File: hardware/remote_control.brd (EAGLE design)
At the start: 19.5 x 100 mm, 52 parts, among them IC1 MCP4726, IC3 REG1117, IC4 TL072D, IC5 LM4041A12DBZ

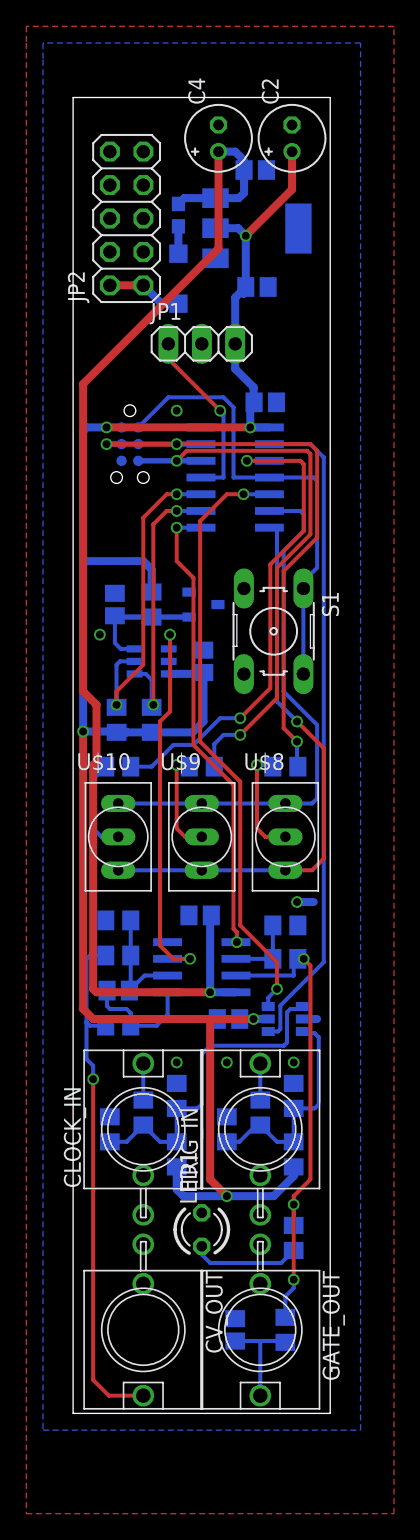
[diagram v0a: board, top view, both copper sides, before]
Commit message: rfsw
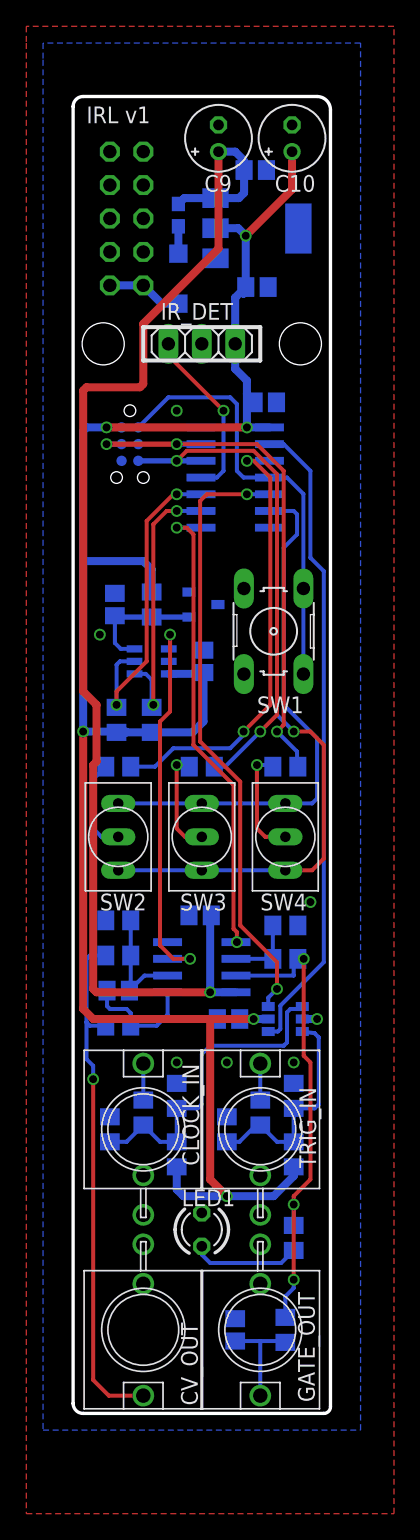
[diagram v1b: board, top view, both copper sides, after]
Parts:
- removed C11, C12: (no value), resistor:C0805
- removed D9: TS4148, jason_eagle6:D0805
- added C3: (no value), resistor:C0805
- added D2: TS4148, jason_eagle6:D0805
- added R3: (no value), rcl:R0805
- C10, C9: device resistor:C0805 -> resistor:E2-5
- C2, C4: device resistor:E2-5 -> resistor:C0805
- IC1: value MCP4726 -> REG1117; device jasons_stuff:SOT23-6 -> burr-brown:SOT223
- IC3: value REG1117 -> LM4041A12DBZ; device burr-brown:SOT223 -> texas:DBZ_R-PDSO-G3
- IC4: value TL072D -> MCP4726; device linear:SO08 -> jasons_stuff:SOT23-6
- IC5: value LM4041A12DBZ -> TL072D; device texas:DBZ_R-PDSO-G3 -> linear:SO08
- R1: value (none) -> 3k
- R14: value 3k -> (none)
- R8: device rcl:R0805 -> resistor:C0805
- moved C10 90.7 mm to (20.2, 96.9), flipped to the top, turned to 90 degrees
- moved C8 70.5 mm to (15.9, 6.35), turned to 270 degrees
- moved C1 64.5 mm to (17.4, 94.5), turned to 0 degrees
- moved R1 49.3 mm to (9.53, 61.5), turned to 90 degrees
- moved R14 49.3 mm to (20.3, 13.3), turned to 270 degrees
- moved R15 48.1 mm to (19.7, 6.35), turned to 90 degrees
- moved C6 47.9 mm to (13.2, 37.8)
- moved C5 37.5 mm to (13.5, 57.1), turned to 90 degrees
- moved C4 36.3 mm to (6.73, 61.5), flipped to the bottom, turned to 270 degrees
- moved C9 36.3 mm to (14.6, 96.9), flipped to the top, turned to 90 degrees
- moved IC1 33.9 mm to (17.5, 90.0), turned to 90 degrees
- moved D4 32.3 mm to (6.99, 49.1), turned to 180 degrees
- moved D7 30.6 mm to (11.4, 19.7), turned to 270 degrees
- moved IC3 28.9 mm to (13.5, 61.5)
- moved R8 28.7 mm to (6.99, 32.1), turned to 0 degrees
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- renumbered FB1 to L1, JP1 to IR_DET, R16 to R2, S1 to SW1, U$1 to IC2, U$10 to SW2, U$6 to IC6, U$8 to SW4, U$9 to SW3
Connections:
- net +12V: now also C1.2, C6.1, C9.+, IC1.3, IC5.8; no longer C12.1, C4.+, C5.2, IC3.3, IC4.8
- net CV_OUT: now also IC4.1, IC5.3; no longer IC1.1, IC4.3
- net GATE_OUT: now also IC5.5; no longer IC4.5
- net GND: now also C10.-, C2.1, C3.1, C4.1, C5.2, C6.2, C7.1, C9.-, D6.A, D8.A, IC1.1, IC3.2, IC4.2, IC5.4, R10.2, R12.2, R4.2, R6.2; no longer C10.1, C12.2, C2.-, C4.-, C5.1, C6.1, C7.2, C9.1, D3.A, D5.A, IC1.2, IC3.1, IC4.4, IC5.2, R13.2, R5.2, R7.2, R9.2
- net N$10: now also R11.1; no longer R4.1
- net N$11: now also D2.A; no longer D7.A
- net N$13: now also IC5.7, R14.1, R15.2, R5.1; no longer IC4.7, R1.1, R10.1, R8.2
- net N$14: now also D7.A, D8.K, R12.1, R13.2; no longer D5.K, D6.A, R6.2, R7.1
- net N$15: now also D3.A; no longer D8.A
- net N$16: now also C8.2, R15.1; no longer C10.2, R8.1
- net N$17: now also IC5.6, R4.1, R5.2; no longer IC4.6, R10.2, R9.1
- net N$18: now also IC5.2, R6.1, R7.2, R8.1; no longer C11.1, IC4.2, R12.2, R13.1
- net N$19: now also R7.1, R9.1; no longer R11.1, R12.1
- net N$20: now also IC5.1, R8.2, R9.2; no longer C11.2, IC4.1, R11.2
- net N$25: now also D4.A; no longer D9.A
- net N$5: now also R14.2; no longer R1.2
- net N$6: now also C4.2, IC3.1, IC4.6, R1.1; no longer C9.2, IC1.6, IC5.1, R14.1
- net N$9: now also R13.1; no longer R6.1
- net SCAN1: now also D2.K; no longer D7.K
- net SCAN2: now also D3.K; no longer D8.K
- net SCAN3: now also D4.K; no longer D9.K
- net SCL: now also IC4.5, R3.1; no longer IC1.5, R15.1
- net SDA: now also IC4.4; no longer IC1.4
- net VDD: now also C10.+, C2.2, C3.2, C5.1, C7.2, D5.K, D7.K, IC1.2, IC4.3, R1.2, R3.2; no longer C1.2, C2.+, C6.2, C7.1, C8.2, D4.K, D6.K, IC1.3, IC3.2, R14.2, R15.2
- net X: now also D5.A, D6.K, R10.1, R11.2; no longer D3.K, D4.A, R4.2, R5.1
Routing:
- net SCAN2: track 42.9 -> 38.1 mm
- net SCAN1: track 44.7 -> 40.6 mm
- net SCAN3: track 37.3 -> 34.0 mm
- net +12V: track 95.5 -> 97.9 mm
- net N$2: track 35.4 -> 33.2 mm
- net GND: track 2.39 -> 1.12 mm, vias 6 -> 7
- net TRIG_IN: track 50.4 -> 49.2 mm
- net VDD: track 151.9 -> 153.1 mm
- net CLOCK_IN: track 45.7 -> 46.6 mm
- net READ2: track 43.4 -> 44.2 mm
- net READ1: track 41.3 -> 40.5 mm
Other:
- board size 19.5 x 100 mm -> 19.6 x 100.1 mm
- board text added: "+12V"
- board text added: "IRL v1"

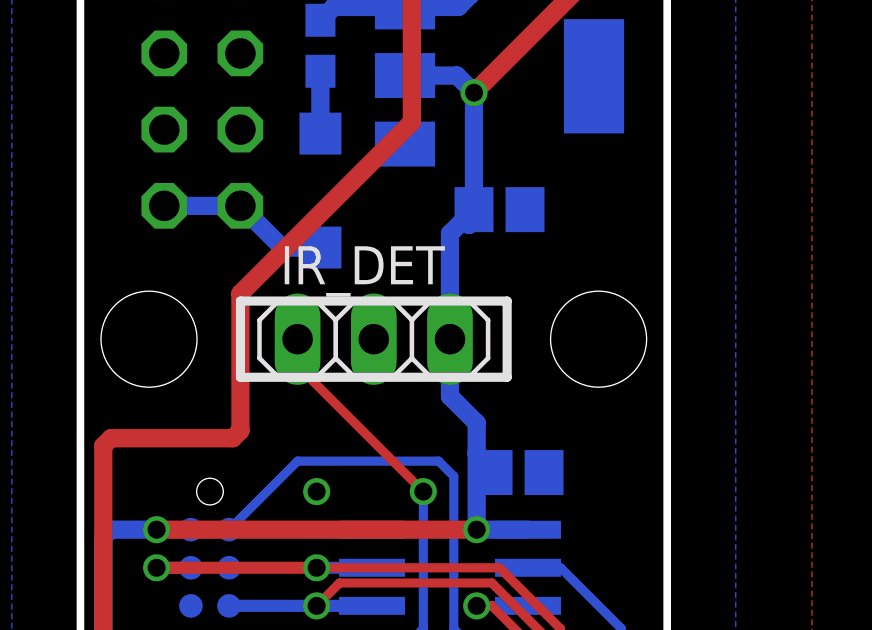
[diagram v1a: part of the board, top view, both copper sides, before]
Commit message: sdf
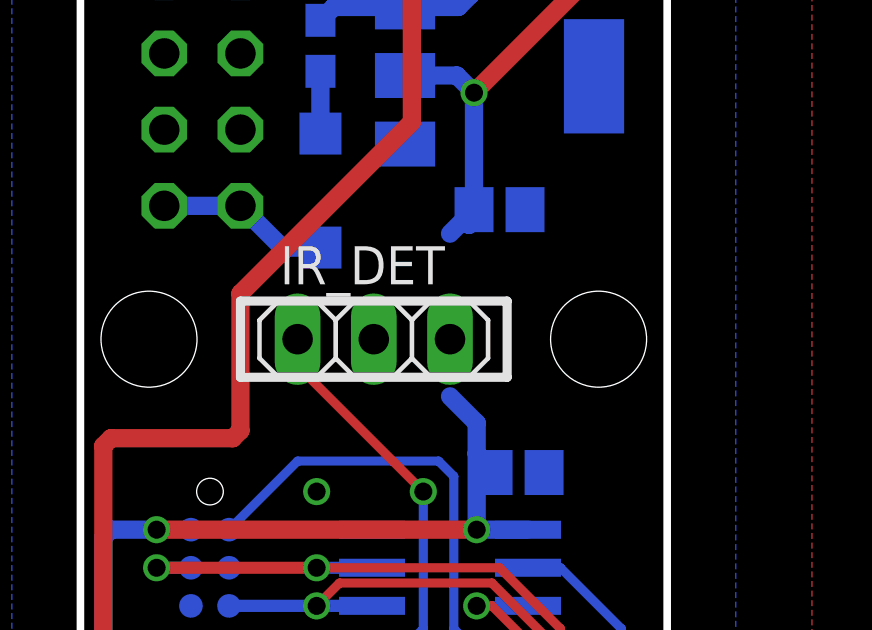
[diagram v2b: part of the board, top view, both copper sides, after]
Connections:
- net GND: now also IR_DET.3; no longer IR_DET.2
- net VDD: now also IR_DET.2; no longer IR_DET.3
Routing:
- net VDD: track 153.1 -> 147.7 mm
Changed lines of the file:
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@@
 <contactref element="IC3" pad="2"/>
 <contactref element="C4" pad="1"/>
-<contactref element="IR_DET" pad="2"/>
 <contactref element="JP2" pad="3"/>
 <contactref element="JP2" pad="7"/>
@@
 <via x="11.43" y="76.2" extent="1-16" drill="0.6"/>
 <via x="22.098" y="29.972" extent="1-16" drill="0.6"/>
+<contactref element="IR_DET" pad="3"/>
+<wire x1="18.249" y1="94.488" x2="20.193" y2="97.917" width="0" layer="19" extent="16-16"/>
+<wire x1="14.605" y1="97.917" x2="18.249" y2="94.488" width="0" layer="19" extent="16-16"/>
+<wire x1="8.89" y1="93.345" x2="14.605" y2="97.917" width="0" layer="19" extent="1-1"/>
+<wire x1="6.35" y1="93.345" x2="8.89" y2="93.345" width="0" layer="19" extent="1-1"/>
+<wire x1="8.89" y1="90.805" x2="8.89" y2="93.345" width="0" layer="19" extent="1-1"/>
+<wire x1="6.35" y1="90.805" x2="6.35" y2="93.345" width="0" layer="19" extent="1-1"/>
+<wire x1="8.89" y1="88.265" x2="8.89" y2="90.805" width="0" layer="19" extent="1-1"/>
+<wire x1="6.35" y1="88.265" x2="6.35" y2="90.805" width="0" layer="19" extent="1-1"/>
+<wire x1="14.3764" y1="87.7824" x2="8.89" y2="88.265" width="0" layer="19" extent="16-16"/>
+<wire x1="18.376" y1="85.598" x2="14.3764" y2="87.7824" width="0" layer="19" extent="16-16"/>
+<wire x1="15.875" y1="81.28" x2="18.376" y2="85.598" width="0" layer="19" extent="16-16"/>
+<wire x1="19.011" y1="76.835" x2="15.875" y2="81.28" width="0" layer="19" extent="16-16"/>
+<wire x1="13.275" y1="74.93" x2="19.011" y2="76.835" width="0" layer="19" extent="16-16"/>
+<wire x1="11.43" y1="76.2" x2="13.275" y2="74.93" width="0" layer="19" extent="16-16"/>
+<wire x1="8.509" y1="73.66" x2="11.43" y2="76.2" width="0" layer="19" extent="16-16"/>
+<wire x1="6.731" y1="62.318" x2="8.509" y2="73.66" width="0" layer="19" extent="16-16"/>
+<wire x1="5.588" y1="59.182" x2="6.731" y2="62.318" width="0" layer="19" extent="16-16"/>
+<wire x1="12.362" y1="62.418" x2="6.731" y2="62.318" width="0" layer="19" extent="16-16"/>
+<wire x1="16.5354" y1="62.6872" x2="12.362" y2="62.418" width="0" layer="19" extent="16-16"/>
+<wire x1="13.462" y1="58" x2="12.362" y2="62.418" width="0" layer="19" extent="16-16"/>
+<wire x1="10.825" y1="57.15" x2="13.462" y2="58" width="0" layer="19" extent="16-16"/>
+<wire x1="16.5354" y1="56.1848" x2="13.462" y2="58" width="0" layer="19" extent="16-16"/>
+<wire x1="21.59" y1="38.862" x2="16.5354" y2="56.1848" width="0" layer="19" extent="1-1"/>
+<wire x1="20.635" y1="37.084" x2="21.59" y2="38.862" width="0" layer="19" extent="16-16"/>
+<wire x1="20.975" y1="29.972" x2="20.635" y2="37.084" width="0" layer="19" extent="16-16"/>
+<wire x1="20.32" y1="26.67" x2="20.975" y2="29.972" width="0" layer="19" extent="16-16"/>
+<wire x1="20.32" y1="25.08" x2="20.32" y2="26.67" width="0" layer="19" extent="16-16"/>
+<wire x1="15.24" y1="26.67" x2="20.32" y2="26.67" width="0" layer="19" extent="1-1"/>
+<wire x1="14.517" y1="29.972" x2="15.24" y2="26.67" width="0" layer="19" extent="16-16"/>
+<wire x1="11.43" y1="26.67" x2="15.24" y2="26.67" width="0" layer="19" extent="1-1"/>
+<wire x1="11.43" y1="25.08" x2="11.43" y2="26.67" width="0" layer="19" extent="16-16"/>
+<wire x1="15.24" y1="22.54" x2="15.24" y2="26.67" width="0" layer="19" extent="16-16"/>
+<wire x1="6.35" y1="22.54" x2="11.43" y2="25.08" width="0" layer="19" extent="16-16"/>
+<wire x1="10.735" y1="35.814" x2="14.517" y2="29.972" width="0" layer="19" extent="16-16"/>
+<wire x1="12.358" y1="37.846" x2="10.735" y2="35.814" width="0" layer="19" extent="16-16"/>
+<wire x1="6.035" y1="37.465" x2="10.735" y2="35.814" width="0" layer="19" extent="16-16"/>
+<wire x1="13.335" y1="15.24" x2="15.24" y2="22.54" width="0" layer="19" extent="16-16"/>
+<wire x1="17.78" y1="15.09" x2="13.335" y2="15.24" width="0" layer="19" extent="1-1"/>
+<wire x1="17.78" y1="12.85" x2="17.78" y2="15.09" width="0" layer="19" extent="1-1"/>
+<wire x1="8.89" y1="15.09" x2="13.335" y2="15.24" width="0" layer="19" extent="1-1"/>
+<wire x1="8.89" y1="12.85" x2="8.89" y2="15.09" width="0" layer="19" extent="1-1"/>
+<wire x1="15.875" y1="7.2" x2="17.78" y2="12.85" width="0" layer="19" extent="16-16"/>
 </signal>
 <signal name="SCL">
@@
 </signal>
 <signal name="VDD">
-<contactref element="IR_DET" pad="3"/>
 <contactref element="J1" pad="2"/>
 <contactref element="IC2" pad="1"/>
@@
 <wire x1="16.51" y1="85.09" x2="16.51" y2="85.432" width="0.6096" layer="16"/>
 <wire x1="16.51" y1="85.432" x2="16.676" y2="85.598" width="0.6096" layer="16"/>
-<wire x1="15.875" y1="81.28" x2="15.875" y2="84.797" width="0.6096" layer="16"/>
 <wire x1="15.875" y1="84.797" x2="16.676" y2="85.598" width="0.6096" layer="16"/>
-<wire x1="15.875" y1="81.28" x2="15.875" y2="79.375" width="0.6096" layer="16"/>
 <wire x1="17.272" y1="76.874" x2="17.311" y2="76.835" width="0.6096" layer="16"/>
 <wire x1="16.764" y1="74.93" x2="16.764" y2="77.47" width="0.6096" layer="16"/>
@@
 <wire x1="17.018" y1="76.542" x2="17.018" y2="77.216" width="0.6096" layer="16"/>
 <wire x1="17.018" y1="77.216" x2="16.764" y2="77.47" width="0.6096" layer="16"/>
+<contactref element="IR_DET" pad="2"/>
+<wire x1="13.335" y1="81.28" x2="15.875" y2="84.797" width="0" layer="19" extent="16-16"/>
+<wire x1="15.875" y1="79.375" x2="13.335" y2="81.28" width="0" layer="19" extent="16-16"/>
 </signal>
 <signal name="IR_RX">
